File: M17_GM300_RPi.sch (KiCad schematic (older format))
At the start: 44 parts, among them J1 RJ45, J2 DB9_Female, J3 RPi_SND, J4 Conn_01x20_Female, J5 Conn_01x20_Female, J6 Conn_01x02_Female, Q1 BSS123, Q2 BSS123, Q3 BSS123, U1 4066, U2 LM386, U3 MCP6001U

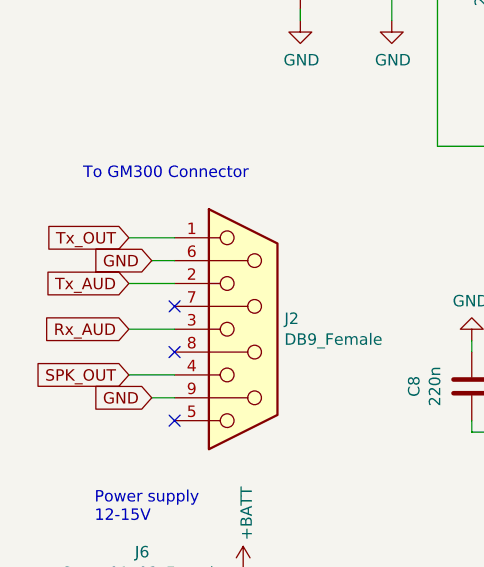
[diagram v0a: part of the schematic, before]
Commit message: fixin' labels
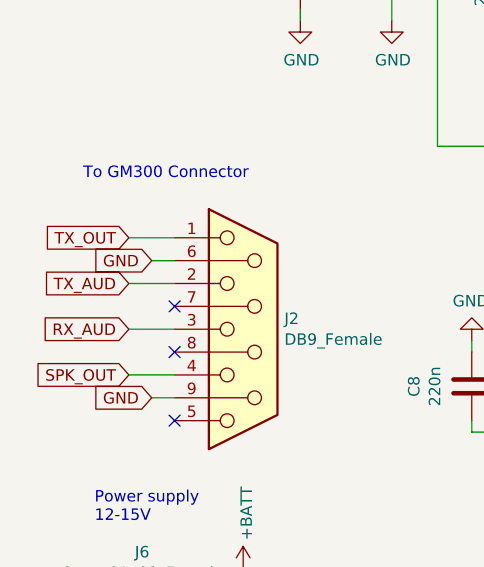
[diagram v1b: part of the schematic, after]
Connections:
- net Rx_AUD is gone; now on net RX_AUD: J2.3
- net Tx_AUD is gone; now on net TX_AUD: J2.2
- net Tx_OUT is gone; now on net TX_OUT: J2.1
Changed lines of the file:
@@
 $EndComp
 Text GLabel 950  5550 0    50   Input ~ 0
-Tx_OUT
+TX_OUT
 Text GLabel 950  5750 0    50   Input ~ 0
-Tx_AUD
+TX_AUD
 Text GLabel 950  5950 0    50   Input ~ 0
-Rx_AUD
+RX_AUD
 Text GLabel 950  6150 0    50   Input ~ 0
 SPK_OUT
